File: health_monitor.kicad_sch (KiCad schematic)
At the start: 0 parts

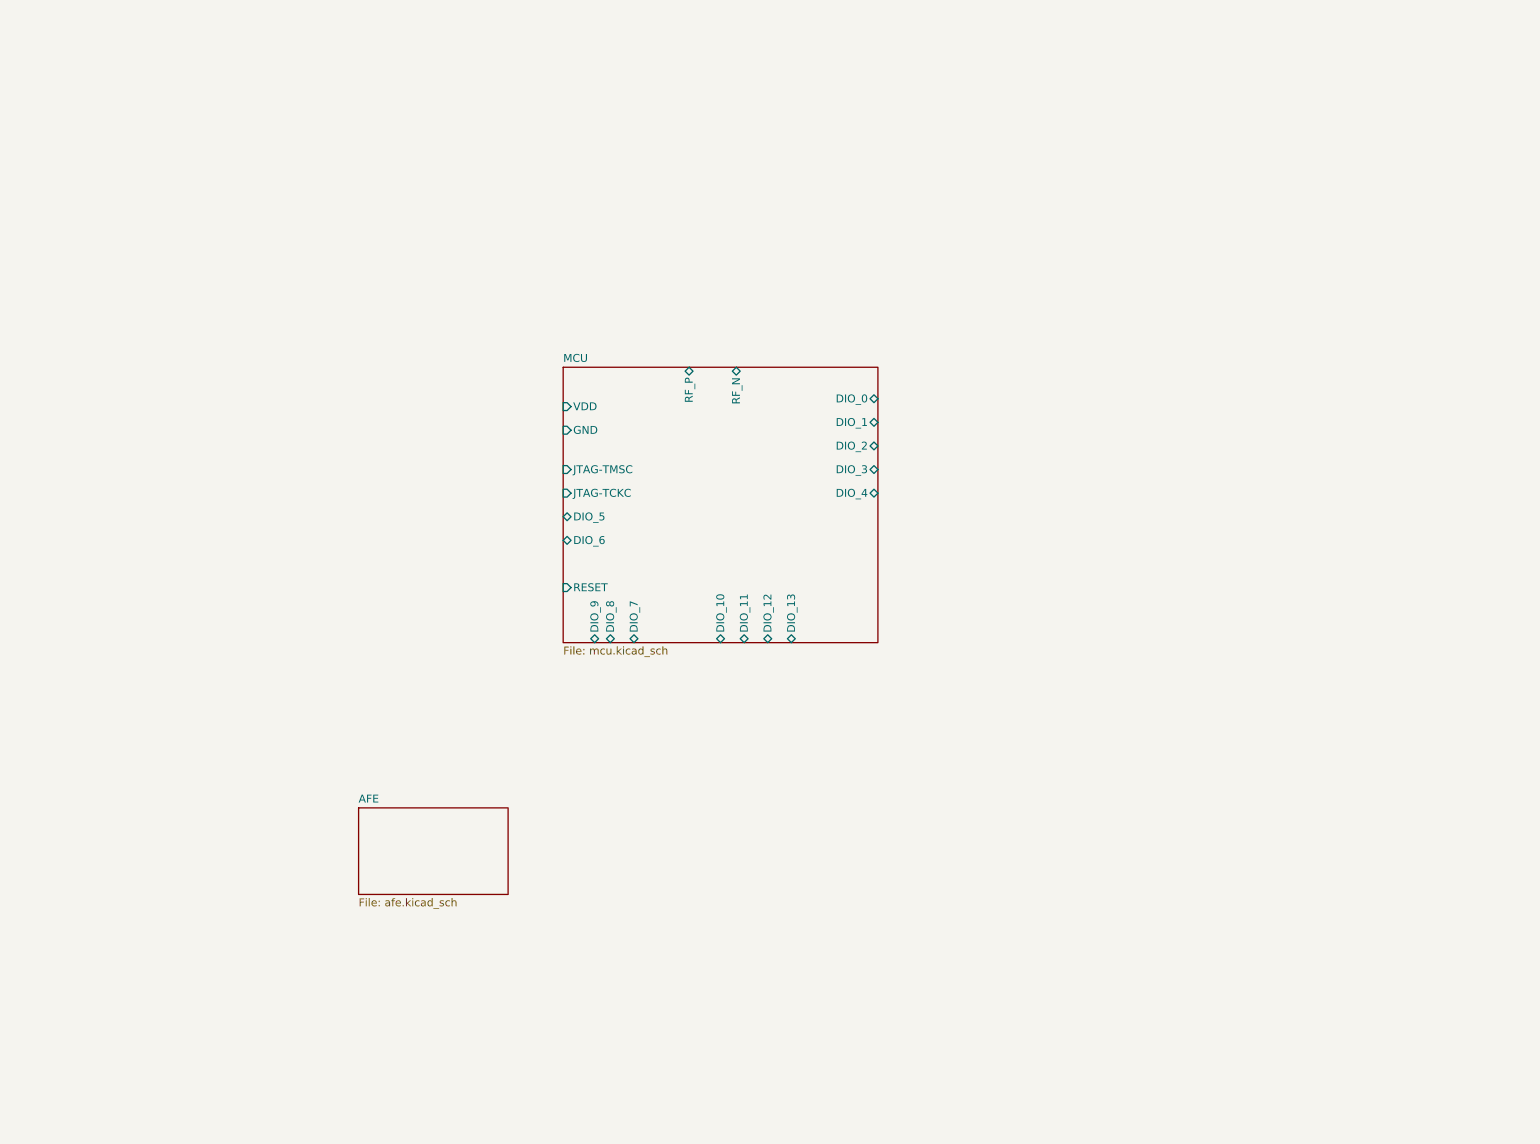
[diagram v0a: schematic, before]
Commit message: schematic 90%
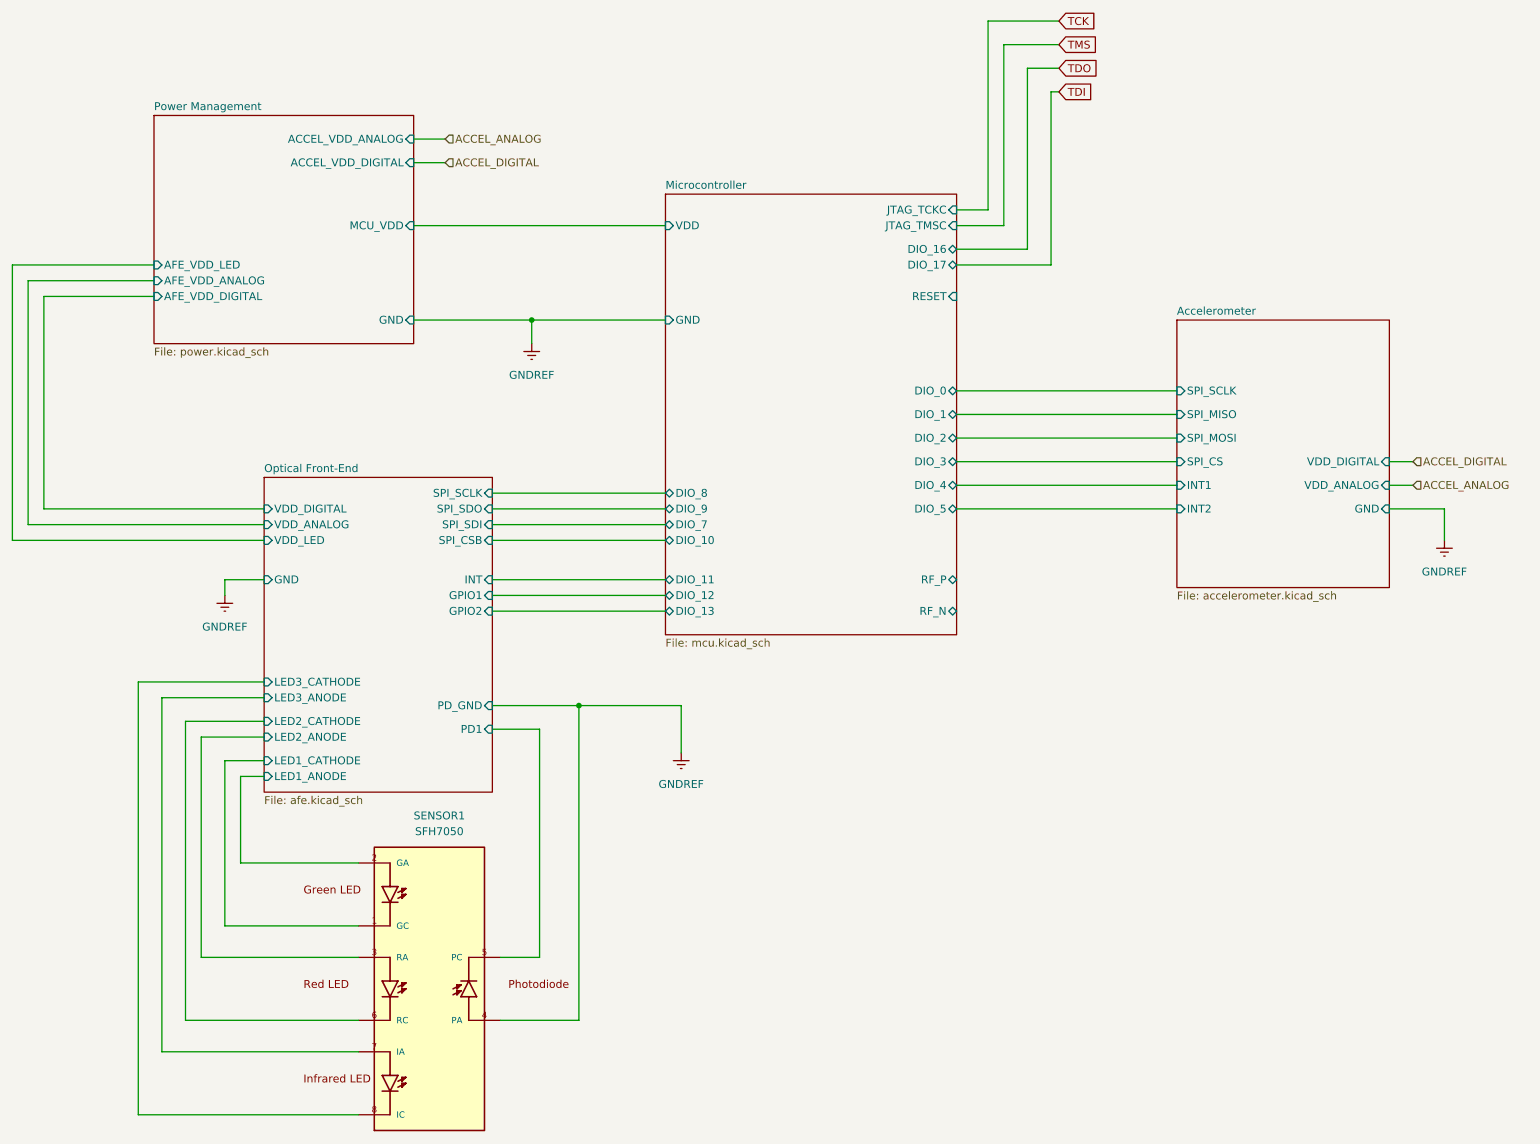
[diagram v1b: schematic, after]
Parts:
- added SENSOR1: SFH7050, SFH7050:OSRAM_SFH7050, symbol ProjectSymbols:SFH7050
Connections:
- new net GNDREF: SENSOR1.4 (PA)
- new net Optical Front-End/LED1_ANODE: SENSOR1.2 (GA)
- new net Optical Front-End/LED1_CATHODE: SENSOR1.1 (GC)
- new net Optical Front-End/LED2_ANODE: SENSOR1.3 (RA)
- new net Optical Front-End/LED2_CATHODE: SENSOR1.6 (RC)
- new net Optical Front-End/LED3_ANODE: SENSOR1.7 (IA)
- new net Optical Front-End/LED3_CATHODE: SENSOR1.8 (IC)
- new net Optical Front-End/PD1: SENSOR1.5 (PC)
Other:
- sheet AFE renamed Optical Front-End
- sheet MCU renamed Microcontroller
- added sheet Accelerometer (accelerometer.kicad_sch)
- added sheet Power Management (power.kicad_sch)
- sheet Microcontroller ports: added DIO_16, DIO_17, JTAG_TCKC, JTAG_TMSC; removed DIO_6, JTAG-TCKC, JTAG-TMSC
- sheet Optical Front-End ports: added GND, GPIO1, GPIO2, INT, LED1_ANODE, LED1_CATHODE, LED2_ANODE, LED2_CATHODE, LED3_ANODE, LED3_CATHODE, PD1, PD_GND, SPI_CSB, SPI_SCLK, SPI_SDI, SPI_SDO, VDD_ANALOG, VDD_DIGITAL, VDD_LED; removed none
- company: (none) -> Guardian Health Inc.
- title: (none) -> Wearable Vital Monitor
